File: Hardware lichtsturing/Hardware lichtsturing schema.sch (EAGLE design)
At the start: 18 parts, among them IC1 LM555N, Q1 TIP41C, X1 Ingang

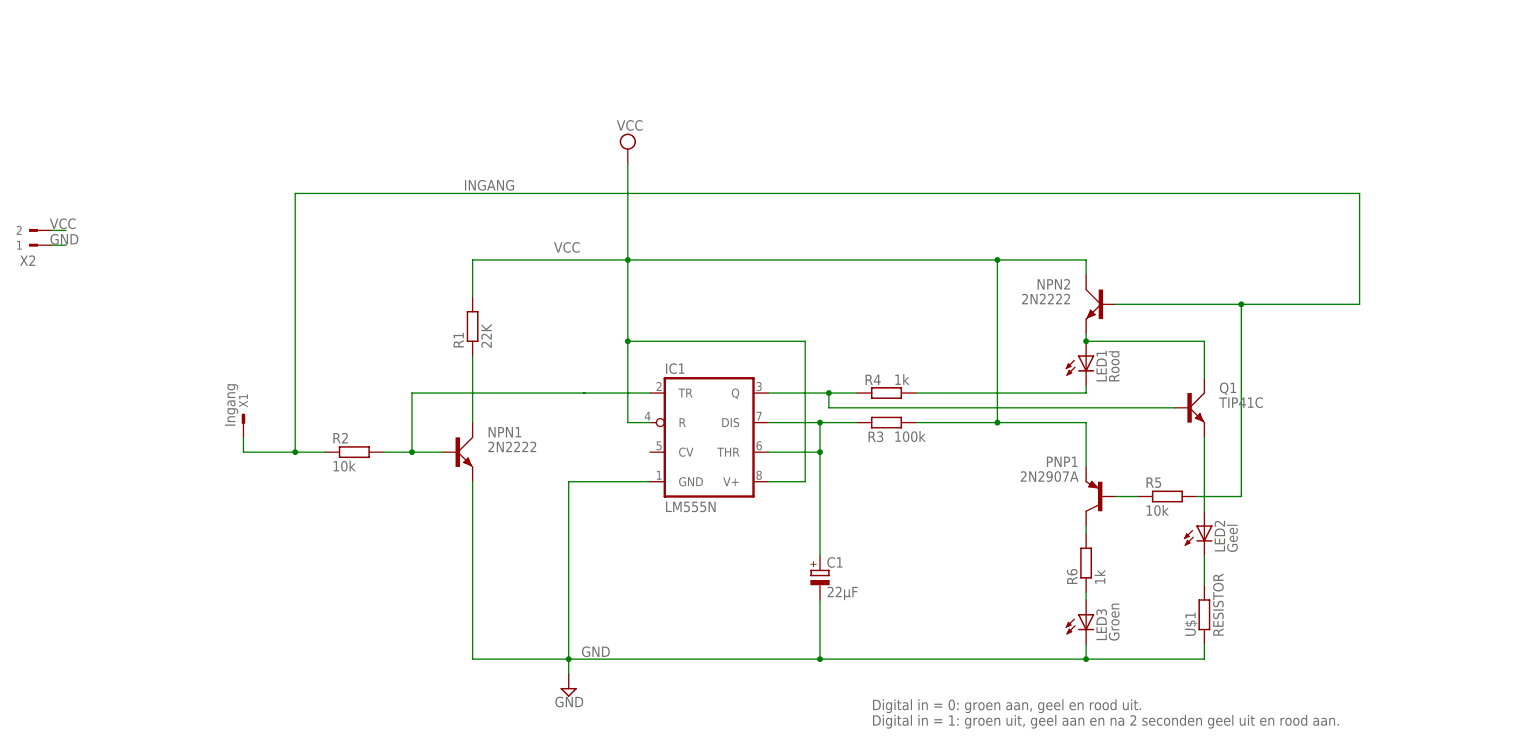
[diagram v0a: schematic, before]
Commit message: Schema lichtsturing, library eindbord, Logboek
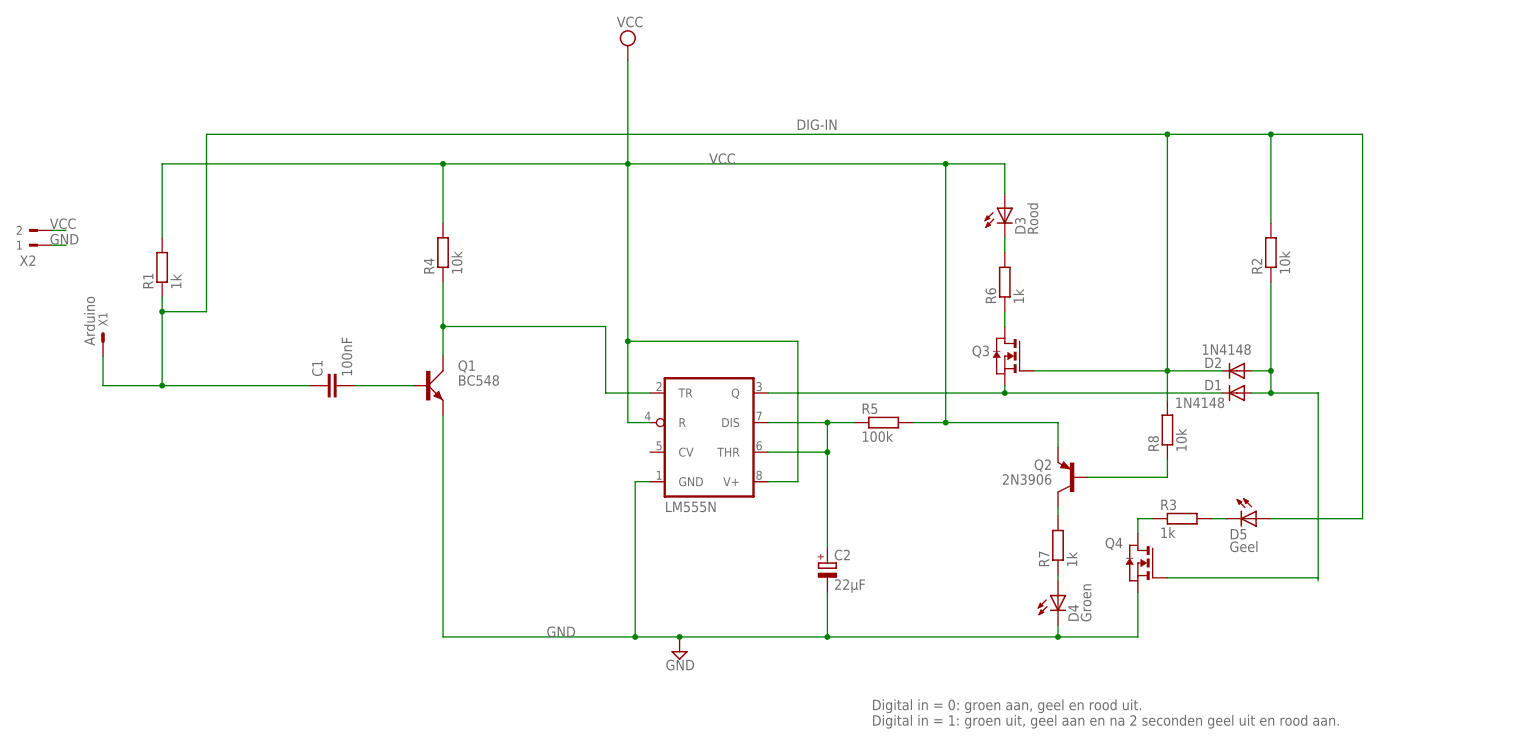
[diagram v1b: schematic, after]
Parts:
- removed LED1: Rood, Hardware lichtsturing library:TLLY4400
- removed LED2: Geel, Hardware lichtsturing library:TLLY4400
- removed LED3: Groen, Hardware lichtsturing library:TLLY4400
- removed NPN1, NPN2: 2N2222, Hardware lichtsturing library:TIP41C
- removed PNP1: 2N2907A, Hardware lichtsturing library:BC307
- removed U$1: RESISTOR, Hardware lichtsturing library:RESISTOR
- added C2: 22µF, Hardware lichtsturing library:ELCO
- added D1, D2: 1N4148, Hardware lichtsturing library:1N4148DO35-7
- added D3: Rood, Hardware lichtsturing library:TLLY4400
- added D4: Groen, Hardware lichtsturing library:TLLY4400
- added D5: Geel, Hardware lichtsturing library:TLLY4400
- added Q2: 2N3906, Hardware lichtsturing library:BC307
- added Q3, Q4: (no value), Hardware lichtsturing library:NMOSE3L
- added R7: 1k, Hardware lichtsturing library:RESISTOR
- added R8: 10k, Hardware lichtsturing library:RESISTOR
- C1: value 22µF -> 100nF; device Hardware lichtsturing library:ELCO -> Hardware lichtsturing library:CAPACITOR
- Q1: value TIP41C -> BC548
- R1: value 22K -> 1k
- R3: value 100k -> 1k
- R4: value 1k -> 10k
- R5: value 10k -> 100k
- X1: value Ingang -> Arduino
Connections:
- removed net INGANG: NPN2.B, R2.1, R5.2, X1.S
- removed net N$2: NPN1.C, R1.1
- new net DIG-IN: C1.1, D2.C, D5.A, Q3.G, R1.1, R2.2, R8.2, X1.S
- new net N$14: Q4.D, R3.1
- new net N$15: D5.C, R3.2
- net GND: now also C2.-, D4.C, Q1.E, Q4.S; no longer C1.-, LED3.C, NPN1.E, U$1.1
- net N$10: now also D3.C, R6.2; no longer LED3.A, R6.1
- net N$11: now also D1.C, IC1.Q, Q3.S; no longer PNP1.B, R5.1
- net N$12: now also D1.A, D2.A, Q4.G, R2.1; no longer LED2.A, Q1.E
- net N$3: now also C1.2, Q1.B; no longer IC1.TR, NPN1.B, R2.2
- net N$4: now also IC1.TR, Q1.C, R4.1; no longer LED2.C, U$1.2
- net N$5: now also C2.+, IC1.DIS, IC1.THR, R5.1; no longer LED1.A, NPN2.E, Q1.C
- net N$6: now also Q2.C, R7.2; no longer LED1.C, R4.2
- net N$7: now also D4.A, R7.1; no longer IC1.Q, Q1.B, R4.1
- net N$8: now also Q2.B, R8.1; no longer C1.+, IC1.DIS, IC1.THR, R3.1
- net N$9: now also Q3.D, R6.1; no longer PNP1.C, R6.2
- net VCC: now also D3.A, Q2.E, R4.2, R5.2; no longer NPN2.C, PNP1.E, R3.2
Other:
- moved on the sheet: Q1, R1, R2, R3, R4, R5, R6, X1
